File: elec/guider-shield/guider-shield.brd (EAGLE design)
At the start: 35.6 x 26.7 mm, 23 parts, among them U2 OPENMV3

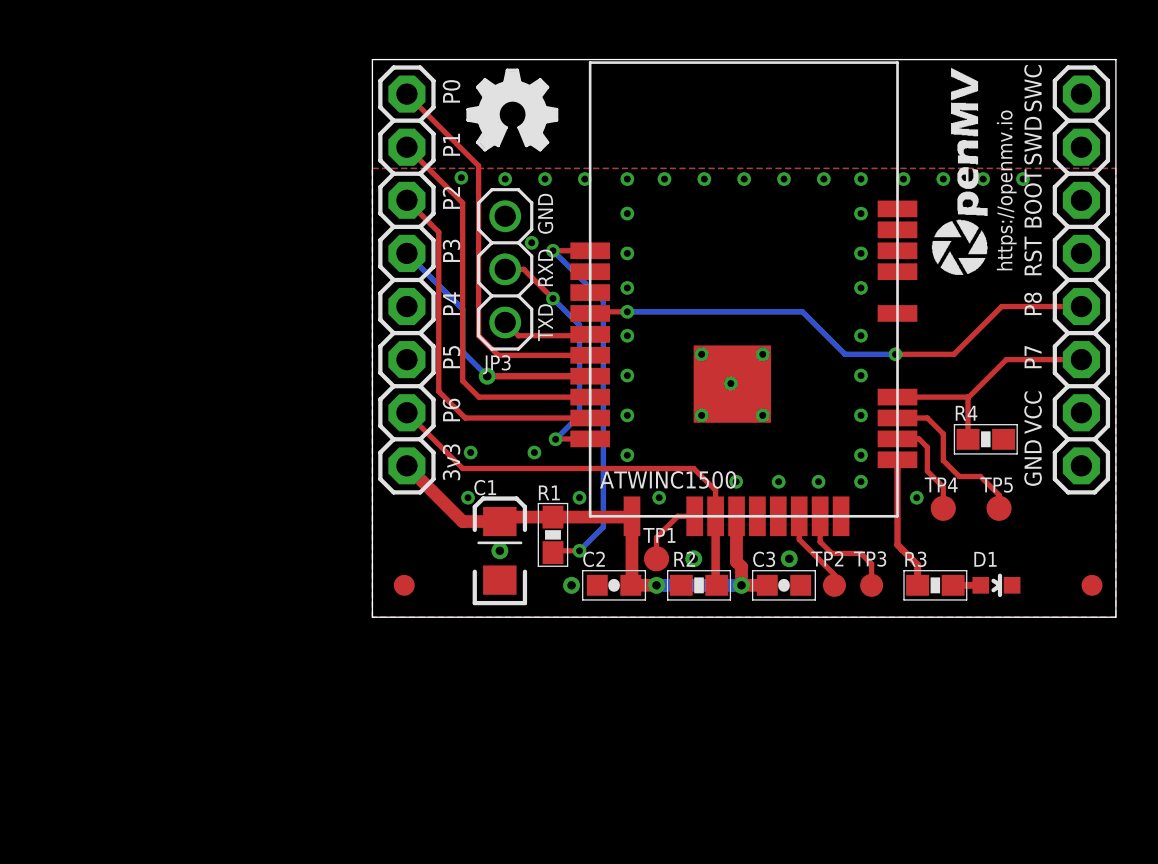
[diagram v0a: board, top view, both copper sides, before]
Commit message: guide-shield almost done
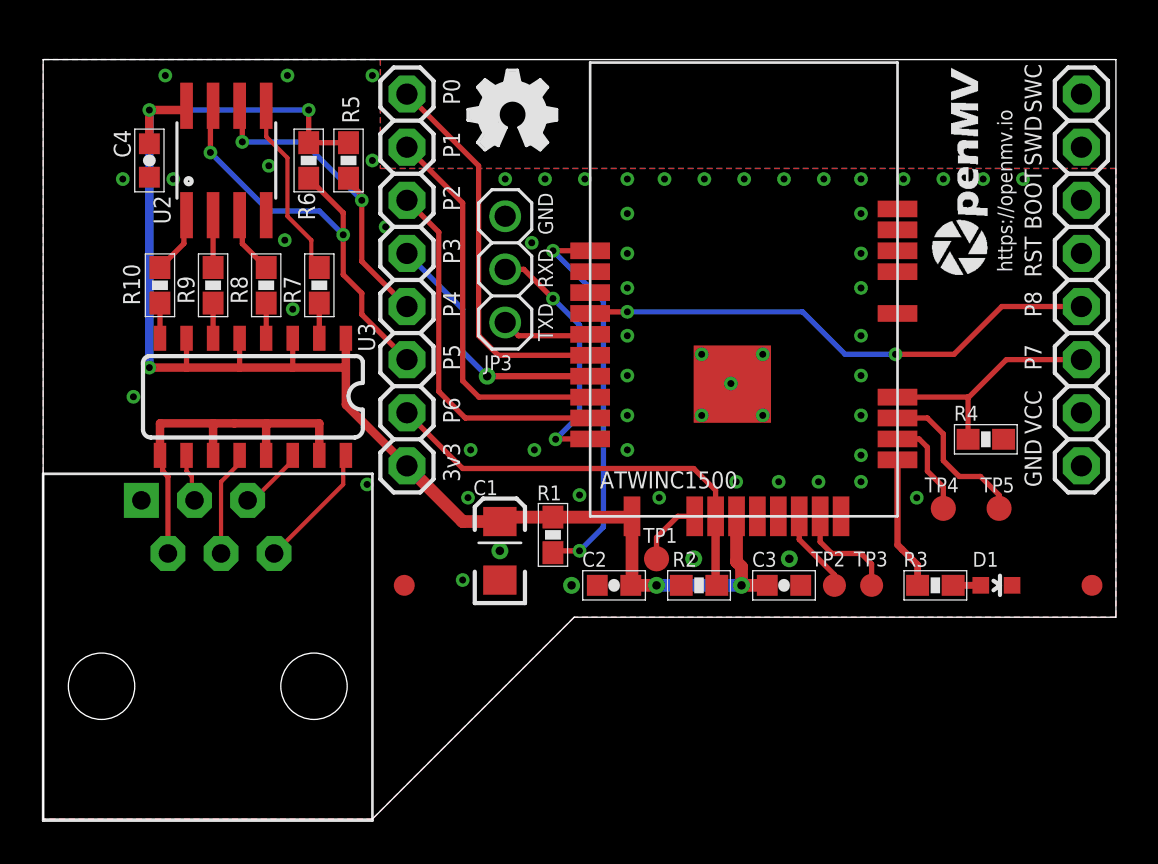
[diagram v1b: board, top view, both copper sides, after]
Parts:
- added C4: 0.1uF, sfe:0603-CAP
- added R10, R7, R8, R9: 220R, sfe:0603-RES
- added R5, R6: 4K7, sfe:0603-RES
- added U3: TLP291, guider-shield:SO016
- added X1: OPENMV3, openmv:OPENMV3
- added X2: MTJ-663X1, guider-shield:MTJ-663X1
- U2: value OPENMV3 -> PCA9536-SO8; device openmv:OPENMV3 -> guider-shield:SO08
- moved U2 17.6 mm to (-6.99, 21.8)
- renumbered U$3 to U1
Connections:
- new net EAST: U3.10, X2.3
- new net N$16: R8.1, U3.4
- new net N$20: R9.1, U3.6
- new net N$21: R10.1, U3.8
- new net N$22: R9.2, U2.2
- new net N$23: R10.2, U2.1
- new net N$24: U3.11, U3.13, U3.15, U3.9, X2.2
- new net N$8: R7.1, U3.2
- new net NORTH: U3.12, X2.4
- new net SCL: R5.1, U2.6, X1.15
- new net SDA: R6.1, U2.7, X1.16
- new net SOUTH: U3.14, X2.5
- new net WEST: U3.16, X2.6
- net 3V3: now also C4.1, R5.2, R6.2, U2.8, U3.1, U3.3, U3.5, U3.7, X1.18; no longer U2.18
- net CHIP_EN: now also X1.17; no longer U2.17
- net GND: now also C4.2, U2.4, X1.28; no longer U2.28
- net IRQ: now also X1.25; no longer U2.25
- net MISO: now also X1.12; no longer U2.12
- net MOSI: now also X1.11; no longer U2.11
- net N$1: now also R7.2, U2.5; no longer U2.15
- net N$2: now also R8.2, U2.3; no longer U2.16
- net RESET: now also X1.26; no longer U2.26
- net SCLK: now also X1.13; no longer U2.13
- net SSEL: now also X1.14; no longer U2.14
- net VIN: now also X1.27; no longer U2.27
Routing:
- net 3V3: track 25.2 -> 73.1 mm, vias 2 -> 5
- net SDA: track 0.00 -> 21.0 mm, vias 0 -> 2
- net N$24: track 0.00 -> 18.6 mm
- net SCL: track 0.00 -> 16.0 mm, vias 0 -> 2
- net N$1: track 0.00 -> 8.79 mm
- net WEST: track 0.00 -> 6.11 mm
- net NORTH: track 0.00 -> 5.06 mm
- net SOUTH: track 0.00 -> 3.20 mm
- net N$23: track 0.00 -> 3.10 mm
- net N$2: track 0.00 -> 3.10 mm
- net N$22: track 0.00 -> 2.50 mm
- net EAST: track 0.00 -> 2.31 mm
- net N$8: track 0.00 -> 1.68 mm
- net N$21: track 0.00 -> 1.68 mm
- net N$20: track 0.00 -> 1.68 mm
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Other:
- board size 35.6 x 26.7 mm -> 51.3 x 36.3 mm
